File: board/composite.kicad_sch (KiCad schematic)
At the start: 23 parts, among them J10 VGA, J6 COMPOSITE, U17 OBVID, Y1 14.318MHz, Y3 25.175MHz

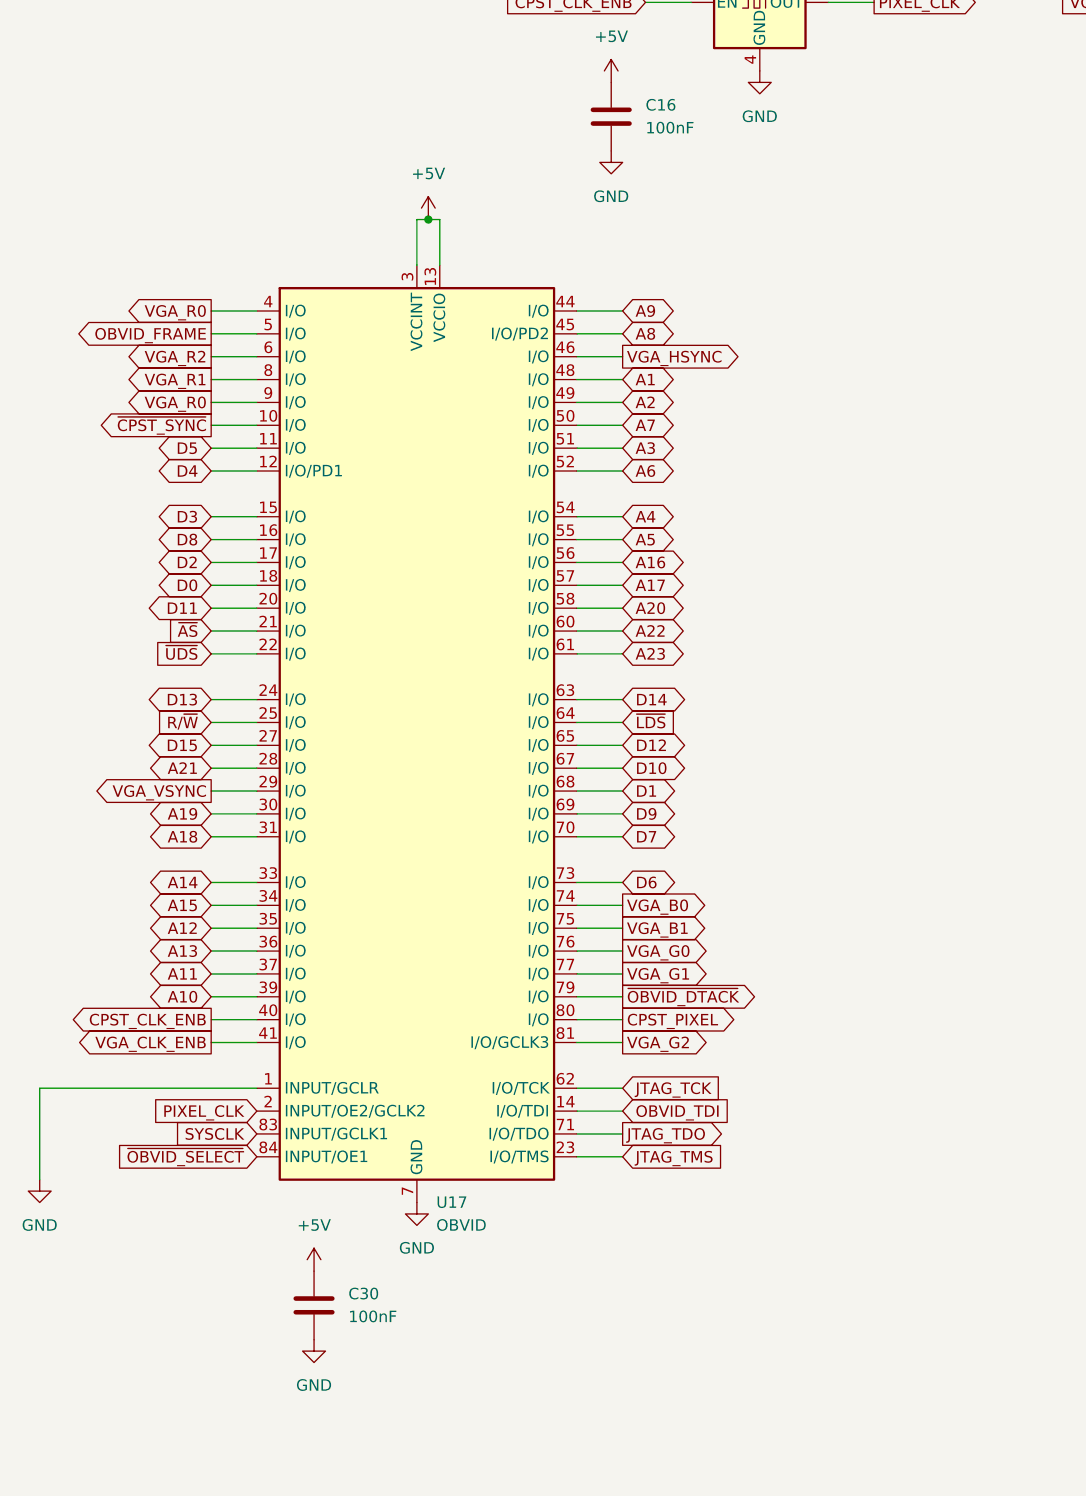
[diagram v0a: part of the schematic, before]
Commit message: checkpoint
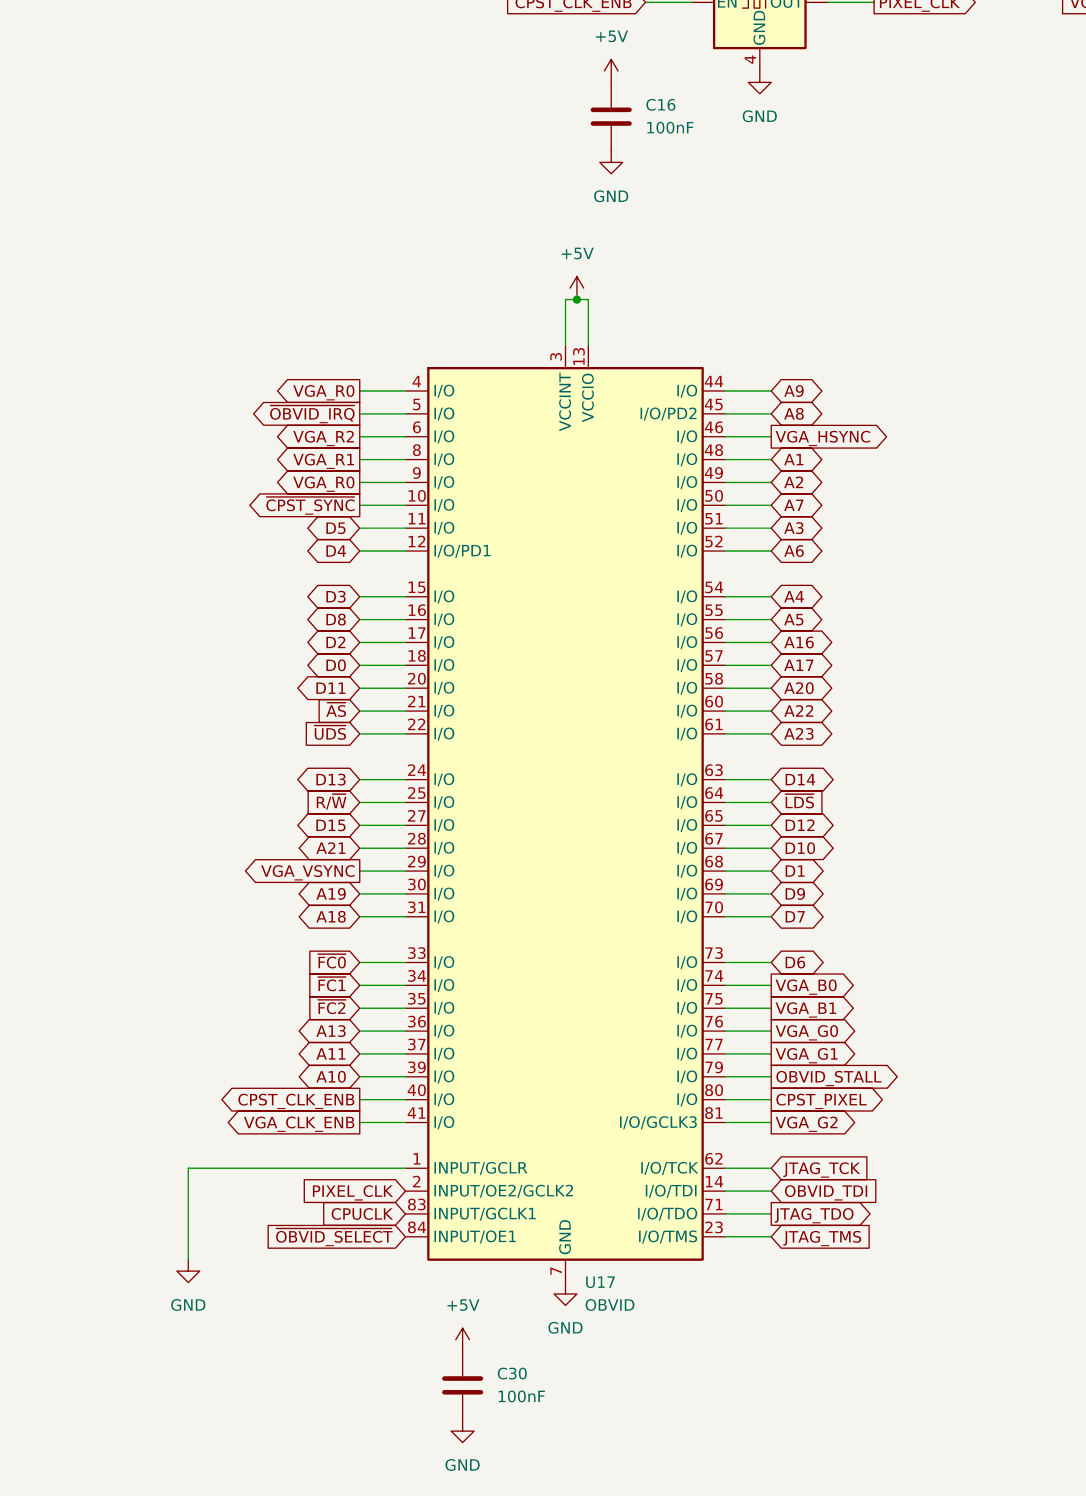
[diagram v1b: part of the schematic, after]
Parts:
- R22, R23: footprint Resistor_SMD:R_0603_1608Metric -> Resistor_THT:R_Axial_DIN0207_L6.3mm_D2.5mm_P10.16mm_Horizontal
- Y3: Digikey https://www.digikey.com/en/products/detail/shenzhen-sctf-electronics/SXOA14-31818A20F30TNN/25795979 -> https://www.digikey.com/en/products/detail/shenzhen-sctf-electronics/SXOA25-175A20F30TNN/25795923?s=N4IgjCBcpgbFoDGUBmBDANgZwKYBoQB7KAbRACYBOAFgAZZKQBdAgBwBcoQBldgJwCWAOwDmIAL4Fq8aCGSR02fEVIUArAHZ6zNp0g9%2BwsZJAMEc1JlwFikMtTBgAHJQ06QHLr0GiJBDRCy8orWKnYgAMwRYGpObiweegY%2BxgSOtObBVsq2ZBHU1OS0GQme%2Bt5GfuBOEZmWSjaqheQalIylSRW%2BJuRq5HUK2Y3h5GDksGDxul6G3QS9tUH1obkUE9TuZcmVPRoySMs5quTUlJMQHTMpVVpuS4MNYWQX0%2BWzqeCOgQcPK6oviSuOzSY2%2BFl%2BR3CMTiERKr22c3AETUG3uIUhz02nXeVRixQG6OGz1OtH6lze1xMYEoLgJQyeIBKPVolH6aPpqwBWy6H1Gagy7Meq16ADpJmoAAQAWQAEgAvLFcACqQgE7AA8igpTg0FgAK58HBVchRJx0oWqKL8yhwwEU4EgAC0YKyFvCsT6zBMjtRP0JDNgESoZO9anNfyh8XE0aAA
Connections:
- net A12 renamed ~{FC2}
- net A14 renamed ~{FC0}
- net A15 renamed ~{FC1}
- net OBVID_FRAME renamed ~{OBVID_IRQ}
- net SYSCLK renamed CPUCLK
- net ~{OBVID_DTACK} renamed OBVID_STALL
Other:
- moved on the sheet: C30, U17

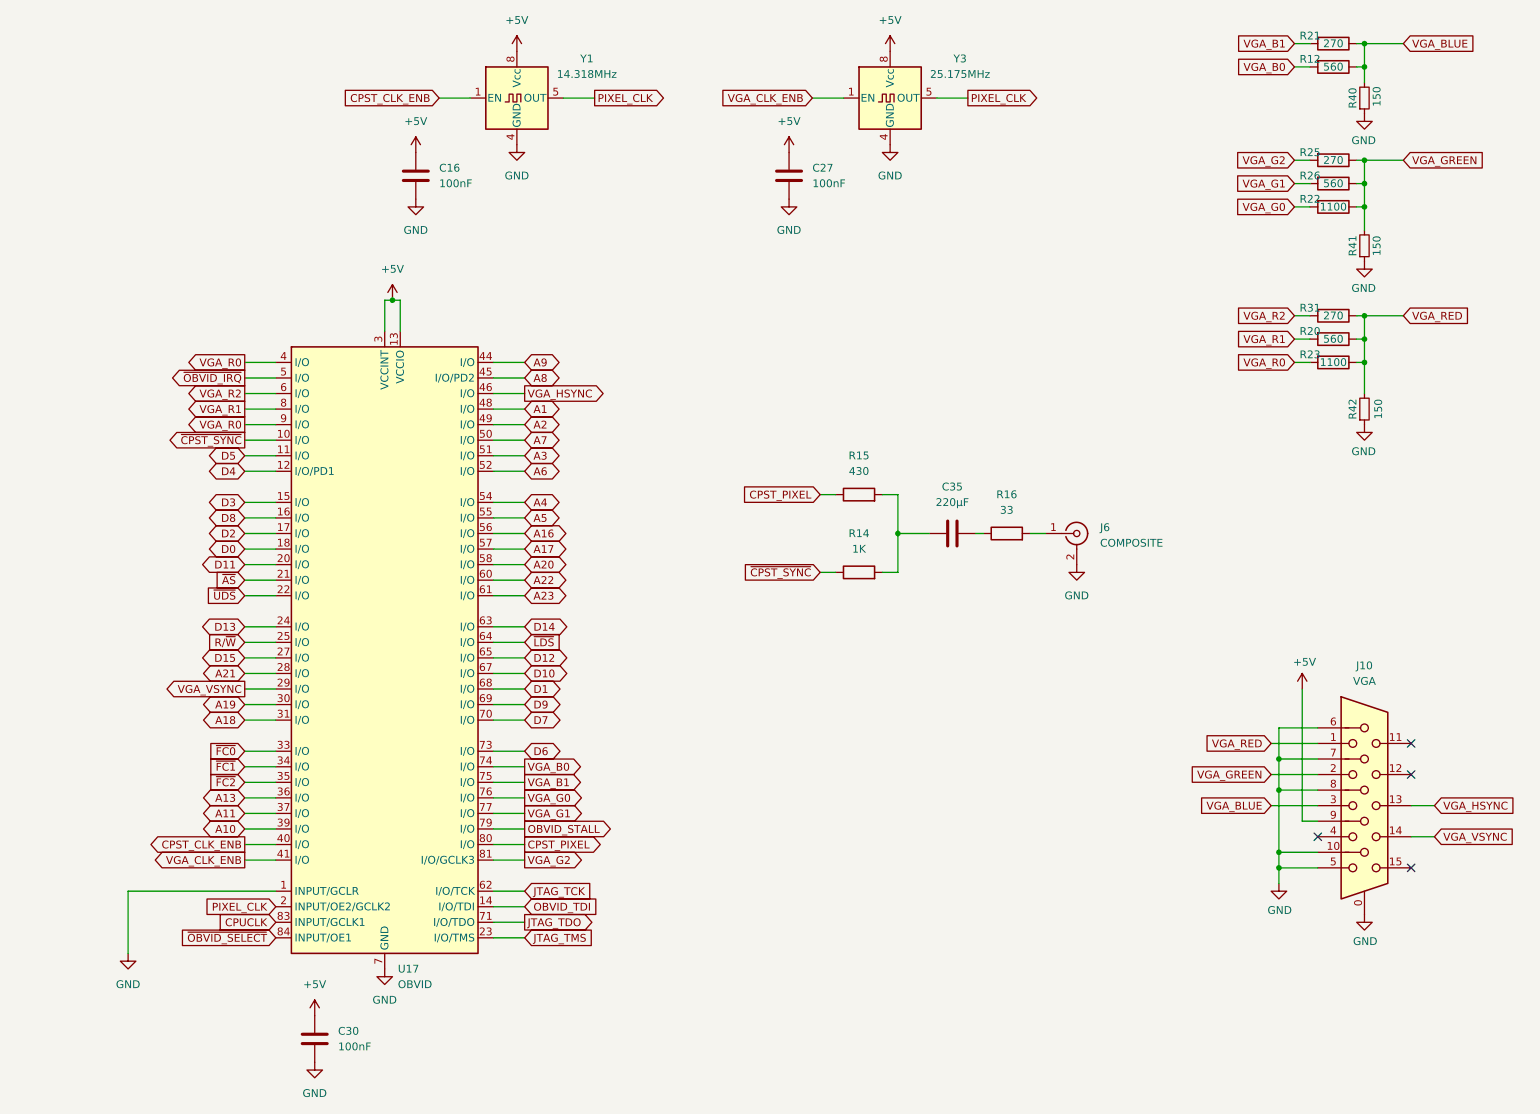
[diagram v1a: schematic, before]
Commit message: Board rev1 PCB complete, already have a spot fix
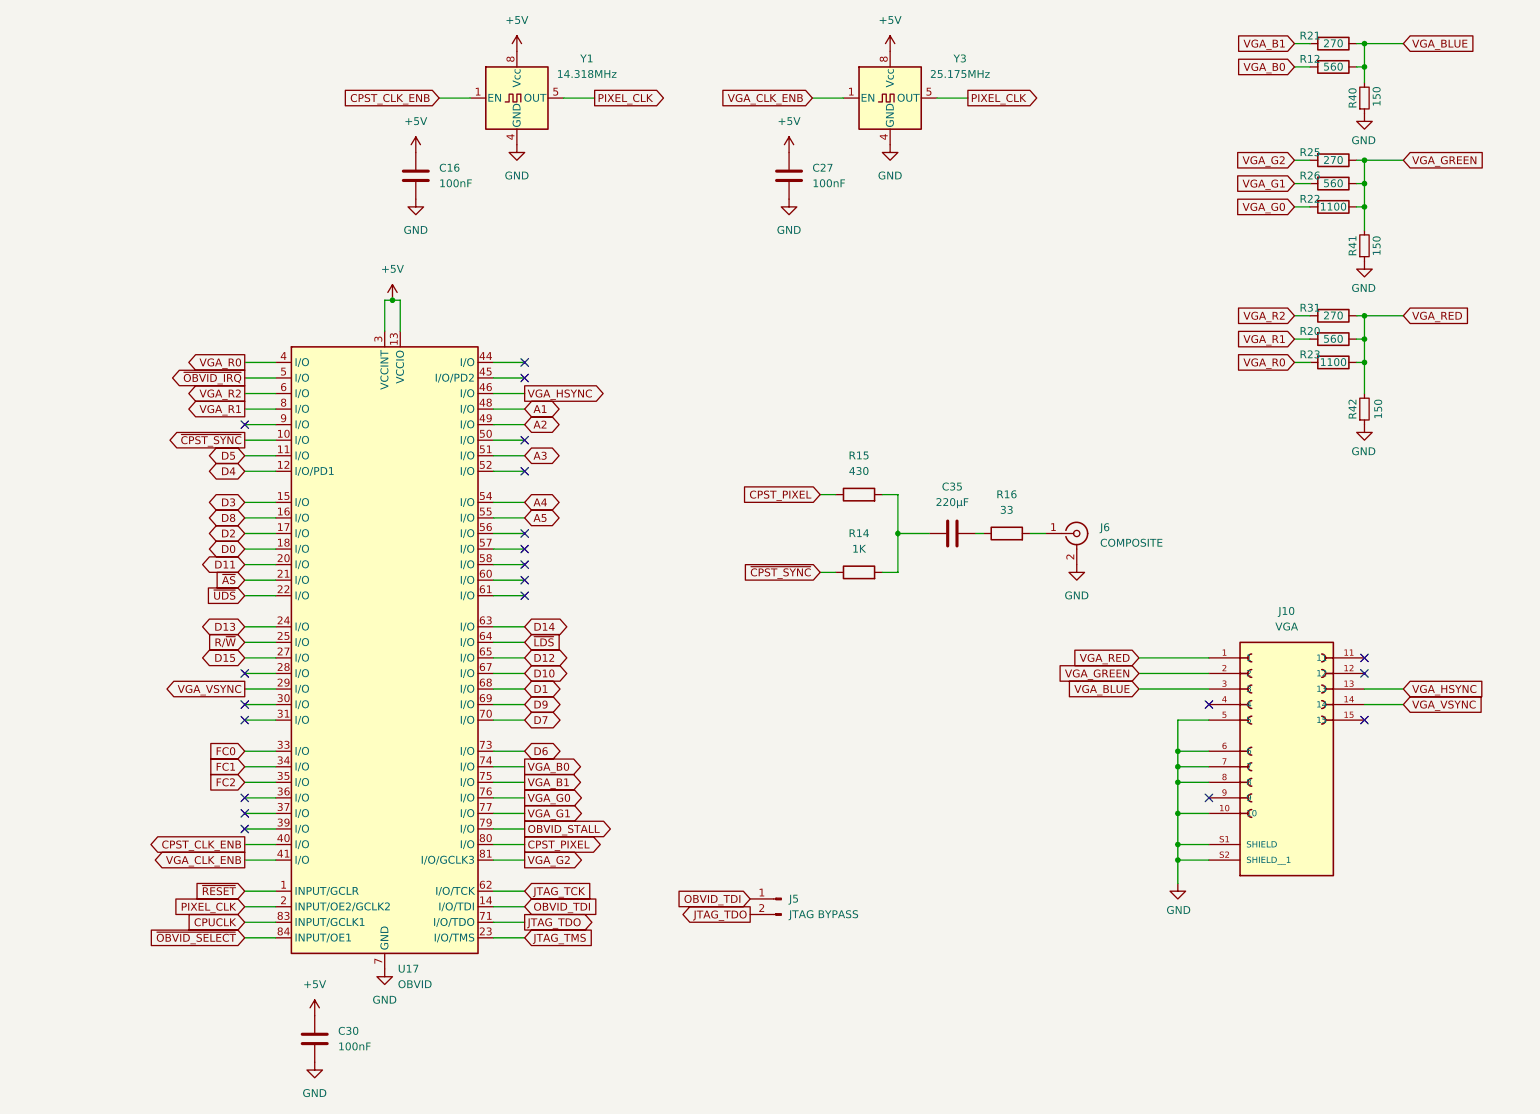
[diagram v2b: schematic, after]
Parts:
- added J5: JTAG BYPASS, Connector_PinHeader_2.54mm:PinHeader_1x02_P2.54mm_Vertical, symbol Connector:Conn_01x02_Pin
- J10: footprint board:HD15-SN-24 -> board:AMPHENOL_ICD15S13E4GX00LF; symbol Connector:DE15_Socket_HighDensity_MountingHoles -> HD15:ICD15S13E4GX00LF; DigiKey (none) -> https://www.digikey.com/en/products/detail/amphenol-cs-fci/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; MANUFACTURER (none) -> Amphenol; MAXIMUM_PACKAGE_HEIGHT (none) -> 12.96mm; PARTREV (none) -> G; STANDARD (none) -> Manufacturer Recommendations
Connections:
- net +5V: no longer J10.9
- net GND: now also J10.S1 (SHIELD), J10.S2 (SHIELD__1); no longer J10.0, U17.1 (INPUT/GCLR)
- net JTAG_TDO: now also J5.2 (Pin_2)
- net OBVID_TDI: now also J5.1 (Pin_1)
- net VGA_R0: no longer U17.9 (I/O)
- net A10: no longer names the net of U17.39 (I/O)
- net A11: no longer names the net of U17.37 (I/O)
- net A13: no longer names the net of U17.36 (I/O)
- net A16: no longer names the net of U17.56 (I/O)
- net A17: no longer names the net of U17.57 (I/O)
- net A18: no longer names the net of U17.31 (I/O)
- net A19: no longer names the net of U17.30 (I/O)
- net A20: no longer names the net of U17.58 (I/O)
- net A21: no longer names the net of U17.28 (I/O)
- net A22: no longer names the net of U17.60 (I/O)
- net A23: no longer names the net of U17.61 (I/O)
- net A6: no longer names the net of U17.52 (I/O)
- net A7: no longer names the net of U17.50 (I/O)
- net A8: no longer names the net of U17.45 (I/O/PD2)
- net A9: no longer names the net of U17.44 (I/O)
- net ~{FC0} renamed FC0
- net ~{FC1} renamed FC1
- net ~{FC2} renamed FC2
- new net ~{RESET}: U17.1 (INPUT/GCLR)
- no-connect marks 4 -> 21
